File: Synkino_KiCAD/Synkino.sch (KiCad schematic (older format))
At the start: 93 parts

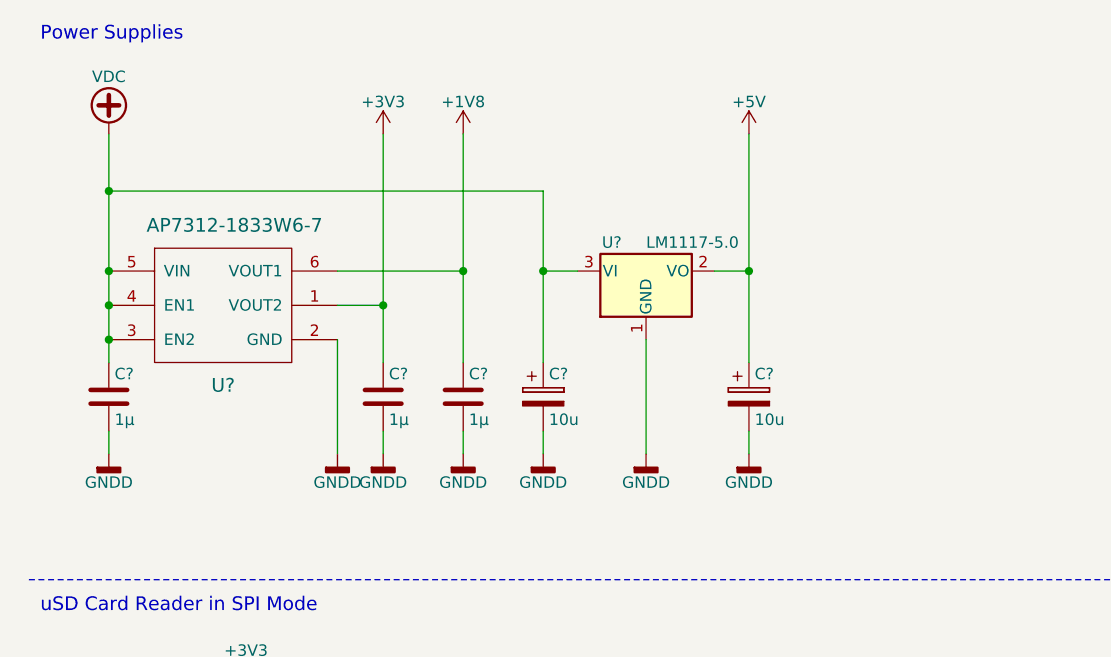
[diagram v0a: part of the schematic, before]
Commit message: Fixing PSU
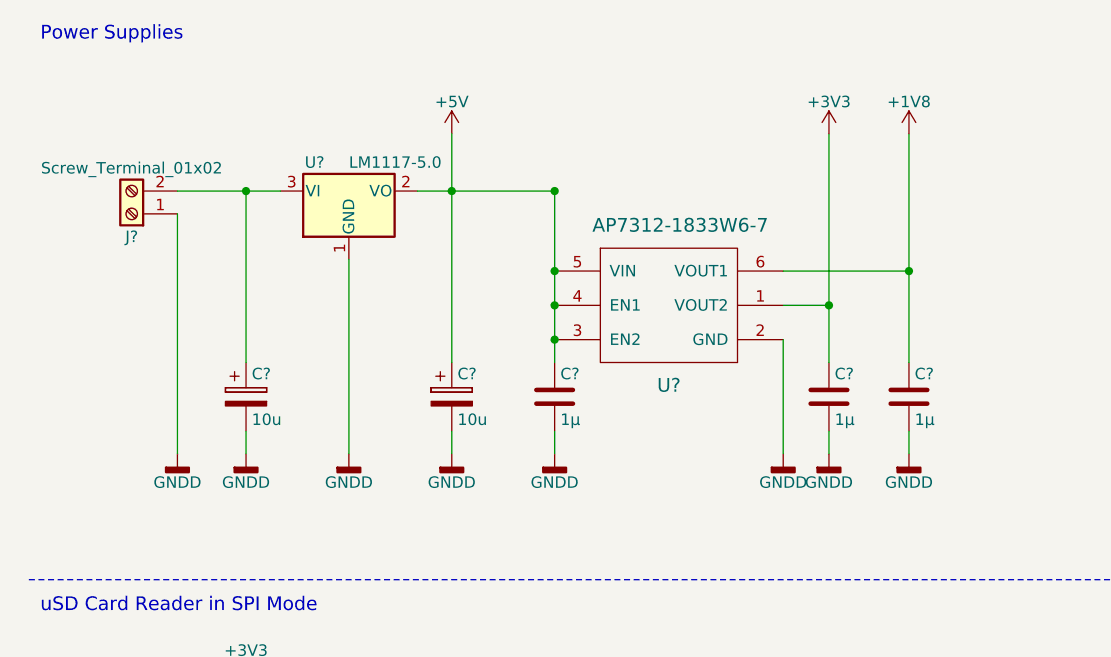
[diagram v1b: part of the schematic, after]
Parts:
- added J?: Screw_Terminal_01x02, symbol Screw_Terminal_01x02
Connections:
- net +5V: now also C?.1, U?.3 (EN2), U?.4 (EN1), U?.5 (VIN)
- net GNDD: now also J?.1 (Pin_1)
- removed net VDC: C?.1, C?.1, U?.3 (EN2), U?.3 (VI), U?.4 (EN1), U?.5 (VIN)
- new net: C?.1, J?.2 (Pin_2), U?.3 (VI)
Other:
- moved on the sheet: C?, U?
